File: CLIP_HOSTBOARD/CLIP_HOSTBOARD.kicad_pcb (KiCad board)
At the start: 2 copper layers, 3 parts, among them J1 505567-0671, U1 Buffer

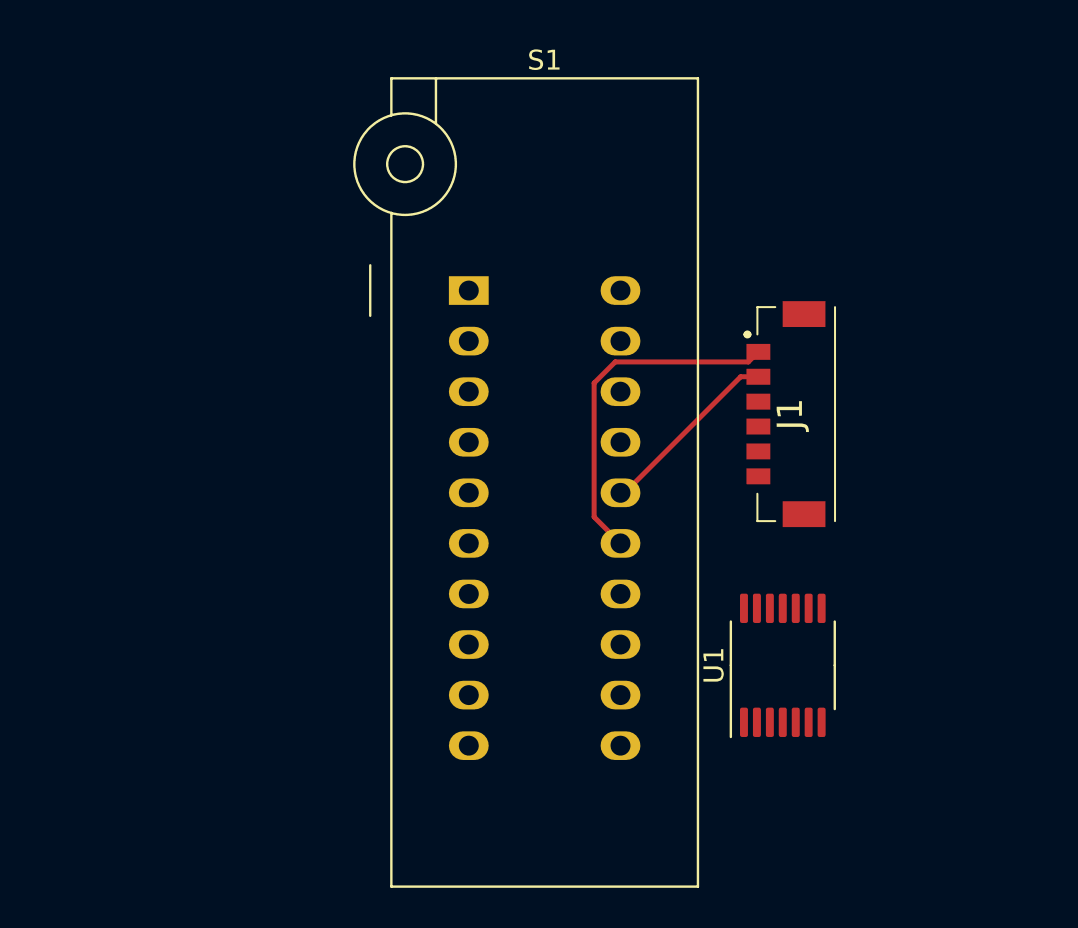
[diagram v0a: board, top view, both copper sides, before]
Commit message: last changes
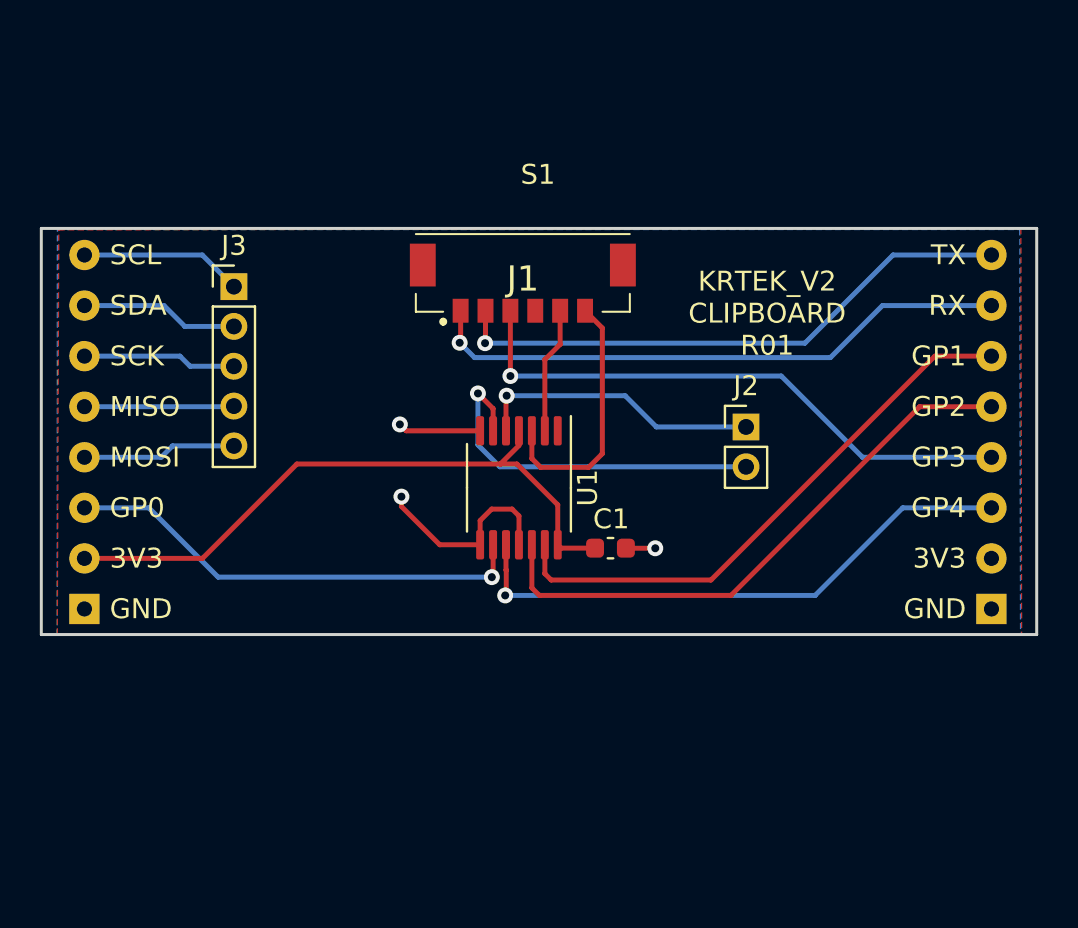
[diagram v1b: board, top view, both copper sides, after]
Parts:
- added C1: 0.1uF, Capacitor_SMD:C_0603_1608Metric, F.Cu at (147.3, 96.6)
- added G***: LOGO, KRTEK_V2:KRTEK_CLIPBOARD, B.Cu at (140.6, 90.7)
- added J2: 1x2_header, Connector_PinHeader_2.00mm:PinHeader_1x02_P2.00mm_Vertical, F.Cu at (154.1, 90.5)
- added J3: 1x5_header, Connector_PinHeader_2.00mm:PinHeader_1x05_P2.00mm_Vertical, F.Cu at (128.4, 83.4)
- S1: footprint Socket:DIP_Socket-20_W4.3_W5.08_W7.62_W10.16_W10.9_3M_220-3342-00-0602J -> hostboard:SOCKET
- moved U1 16.0 mm to (142.7, 93.5), turned to 270 degrees
- moved J1 15.1 mm to (142.9, 83.0), turned to 0 degrees
- moved S1 5.55 mm to (143.6, 79.3)
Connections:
- S1 pad 1: Net-(S1-Pad1) -> SCLFREE
- S1 pad 10: 3V3 -> Net-(S1-Pad10)
- S1 pad 11: Net-(S1-Pad11) -> BFREEIN1
- S1 pad 2: Net-(S1-Pad2) -> SDAFREE
- S1 pad 3: Net-(S1-Pad3) -> SCKFREE
- S1 pad 4: Net-(S1-Pad4) -> MISOFREE
- S1 pad 5: Net-(S1-Pad5) -> MOSIFREE
- S1 pad 6: Net-(S1-Pad6) -> BFREEIN2
- U1 pad 10: Net-(U1-Pad10) -> BFREEIN1
- U1 pad 5: Net-(U1-Pad5) -> BFREEOUT1
- U1 pad 6: Net-(U1-Pad6) -> BFREEOUT2
- U1 pad 9: Net-(U1-Pad9) -> BFREEIN2
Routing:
- net 3V3: track 0.00 -> 32.6 mm
- net HPYRO2: track 0.00 -> 29.3 mm
- net HFREE: track 0.00 -> 29.1 mm, vias 0 -> 1
- net BFREEIN1: track 0.00 -> 28.8 mm, vias 0 -> 1
- net HPYRO1: track 0.00 -> 28.7 mm
- net BFREEIN2: track 0.00 -> 23.6 mm, vias 0 -> 1
- net HTX: track 9.34 -> 28.9 mm, vias 0 -> 1
- net BFREEOUT2: track 0.00 -> 18.7 mm, vias 0 -> 1
- net GND: track 0.00 -> 15.9 mm, vias 0 -> 3
- net BFREEOUT1: track 0.00 -> 14.5 mm, vias 0 -> 1
- net PYRO2: track 0.00 -> 12.9 mm
- net HRX: track 17.5 -> 29.7 mm, vias 0 -> 1
- net SCLFREE: track 0.00 -> 8.17 mm
- net SDAFREE: track 0.00 -> 7.94 mm
- net MOSIFREE: track 0.00 -> 7.74 mm
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- added copper zone on B.Cu, net GND
- added copper zone on F.Cu, net GND
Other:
- board outline added: 50 x 20.4 mm
- board text added: "KRTEK_V2 CLIPBOARD R01"
- board text added: "William Cottier"
